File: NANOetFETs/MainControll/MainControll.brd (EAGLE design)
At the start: 80 x 48.3 mm, 17 parts

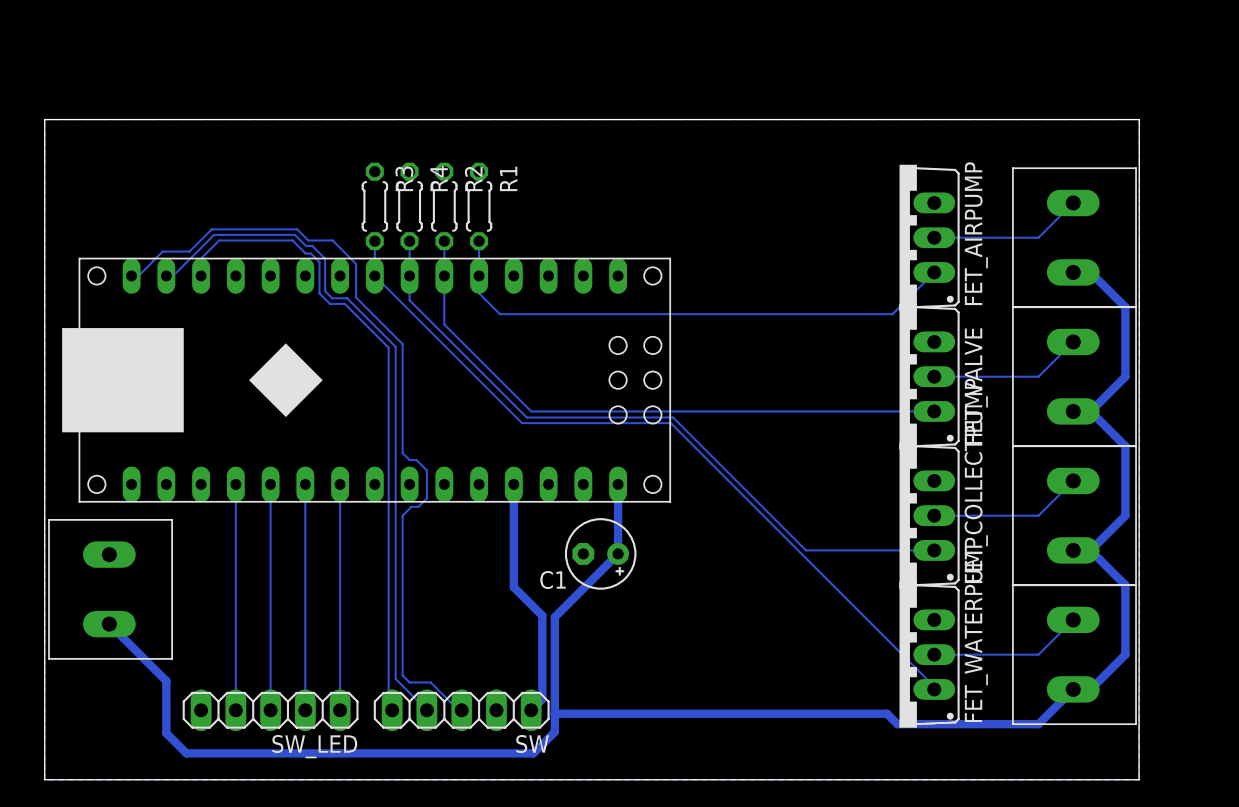
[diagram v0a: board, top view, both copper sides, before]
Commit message: 1st prototype
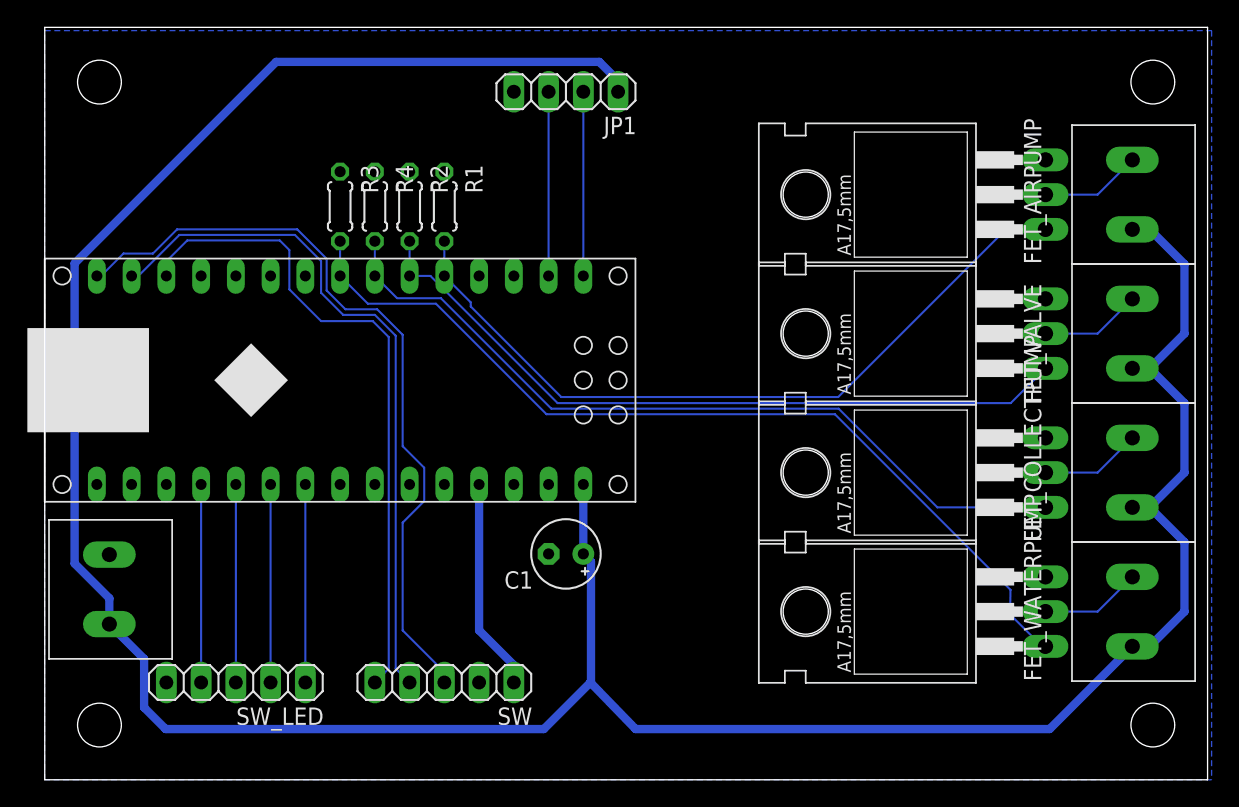
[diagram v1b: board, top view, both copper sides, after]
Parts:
- added JP1: (no value), pinhead:1X04
- FET_AIRPUMP, FET_COLLECTPUMP, FET_VALVE, FET_WATERPUMP: value IRF740 -> 2SK2232; device transistor-power:TO220BV -> Transistor-FET:TO220
- moved FET_COLLECTPUMP 5.34 mm to (66.8, 22.5)
- moved FET_AIRPUMP 5.34 mm to (66.8, 42.8)
- moved FET_VALVE 5.34 mm to (66.8, 32.6)
- moved FET_WATERPUMP 5.34 mm to (66.8, 12.3)
- moved TERMINAL_WATERPUMP 5.34 mm to (79.5, 9.75)
- moved TERMINAL_AIRPUMP 5.34 mm to (79.5, 40.2)
- moved TERMINAL_COLLECTPUMP 5.34 mm to (79.5, 19.9)
- moved TERMINAL_VALVE 5.34 mm to (79.5, 30.1)
- moved SW_LED 3.25 mm to (14.0, 7.11)
- moved R4 2.54 mm to (24.1, 41.9)
- moved C1 2.54 mm to (38.1, 16.5)
- moved R1 2.54 mm to (29.2, 41.9)
- moved R2 2.54 mm to (26.7, 41.9)
- moved R3 2.54 mm to (21.6, 41.9)
- moved U$2 2.54 mm to (21.6, 29.2)
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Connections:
- new net N$1: JP1.3, U$2.RX1
- new net N$2: JP1.2, U$2.TX0
- net +12V: now also JP1.1
- net AIRPUMP: now also FET_AIRPUMP.1; no longer FET_AIRPUMP.G
- net COLPUMP: now also FET_COLLECTPUMP.1; no longer FET_COLLECTPUMP.G
- net GND: now also FET_AIRPUMP.3, FET_COLLECTPUMP.3, FET_VALVE.3, FET_WATERPUMP.3, JP1.4; no longer FET_AIRPUMP.S, FET_COLLECTPUMP.S, FET_VALVE.S, FET_WATERPUMP.S
- net N$10: now also FET_COLLECTPUMP.2; no longer FET_COLLECTPUMP.D
- net N$7: now also FET_AIRPUMP.2; no longer FET_AIRPUMP.D
- net N$8: now also FET_VALVE.2; no longer FET_VALVE.D
- net N$9: now also FET_WATERPUMP.2; no longer FET_WATERPUMP.D
- net VALVE: now also FET_VALVE.1; no longer FET_VALVE.G
- net WATPUMP: now also FET_WATERPUMP.1; no longer FET_WATERPUMP.G
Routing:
- net +12V: track 140.5 -> 216.6 mm
- net AIRPUMP: track 39.0 -> 55.4 mm
- net N$2: track 0.00 -> 13.5 mm
- net N$1: track 0.00 -> 13.5 mm
- net WATPUMP: track 56.1 -> 66.4 mm
- net VALVE: track 44.5 -> 53.9 mm
- net COLPUMP: track 50.2 -> 58.6 mm
- net N$10: track 11.2 -> 7.40 mm
- net N$8: track 11.2 -> 7.40 mm
- net N$7: track 11.2 -> 7.40 mm
- net N$9: track 11.2 -> 7.40 mm
- net +5V: track 17.7 -> 15.5 mm
- net N$14: track 16.5 -> 14.5 mm
- net N$13: track 16.5 -> 14.5 mm
- net N$12: track 16.5 -> 14.5 mm
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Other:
- board size 80 x 48.3 mm -> 85 x 55 mm
